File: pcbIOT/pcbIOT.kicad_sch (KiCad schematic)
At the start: 33 parts, among them IC1 NRF52832-QFAA-G-R7, IC2 TPS62842DGRR, J1 Battery power in, J2 Conn_01x08_Socket, J3 Conn_01x03_Pin, J4 Conn_01x06_Socket, J5 Conn_01x06_Socket, X1 32MHz, X2 32.768kHz

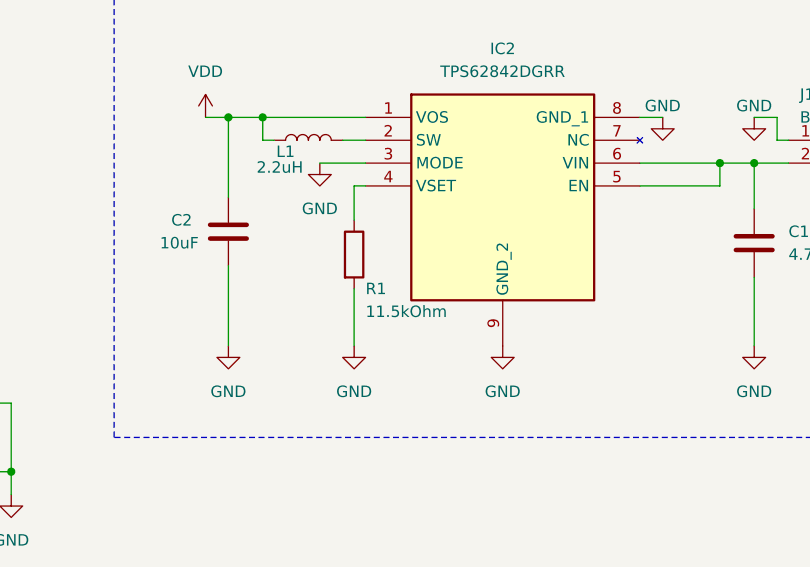
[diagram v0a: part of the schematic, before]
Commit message: pcb bijna af
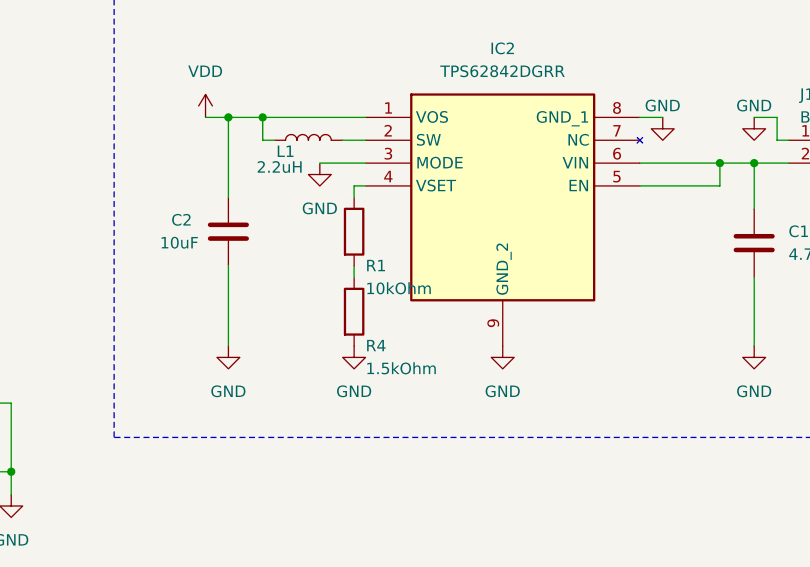
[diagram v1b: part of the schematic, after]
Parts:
- added R4: 1.5kOhm, Resistor_SMD:R_0805_2012Metric_Pad1.20x1.40mm_HandSolder, symbol Device:R
- C1, C10, C11, C12, C13, C14, C15, C2, C3, C4, C5, C6, C7, C8, C9: footprint Capacitor_SMD:C_0603_1608Metric -> Capacitor_SMD:C_0805_2012Metric_Pad1.18x1.45mm_HandSolder
- L4: footprint Inductor_SMD:L_01005_0402Metric_Pad0.57x0.30mm_HandSolder -> Inductor_SMD:L_0805_2012Metric_Pad1.15x1.40mm_HandSolder
- R1: value 11.5kOhm -> 10kOhm; footprint Resistor_SMD:R_0603_1608Metric -> Resistor_SMD:R_0805_2012Metric_Pad1.20x1.40mm_HandSolder
- R2, R3: footprint Resistor_SMD:R_0603_1608Metric -> Resistor_SMD:R_0805_2012Metric_Pad1.20x1.40mm_HandSolder
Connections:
- net GND: now also R4.2; no longer R1.2
- new net: R1.2, R4.1
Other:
- moved on the sheet: R1
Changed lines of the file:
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@@
-    (stroke (width 0) (type default))
-  )
-  (wire (pts (xy 209.55 52.07) (xy 209.55 58.42))
     (stroke (width 0) (type default))
   )
@@
     (stroke (width 0) (type default))
   )
-  (wire (pts (xy 209.55 40.64) (xy 209.55 44.45))
-    (stroke (width 0) (type default))
-  )
   (wire (pts (xy 95.25 58.42) (xy 93.98 58.42))
     (stroke (width 0) (type default))
@@
     (stroke (width 0) (type default))
   )
+  (wire (pts (xy 209.55 49.53) (xy 209.55 50.8))
+    (stroke (width 0) (type default))
+  )
   (wire (pts (xy 212.09 149.86) (xy 214.63 149.86))
     (stroke (width 0) (type default))
@@
   )
   (wire (pts (xy 71.12 93.98) (xy 71.12 83.82))
+    (stroke (width 0) (type default))
+  )
+  (wire (pts (xy 209.55 40.64) (xy 209.55 41.91))
     (stroke (width 0) (type default))
   )
@@
       (effects (font (size 1.27 1.27)) (justify left))
     )
-    (property "Footprint" "Capacitor_SMD:C_0603_1608Metric" (at 74.6252 76.2 0)
+    (property "Footprint" "Capacitor_SMD:C_0805_2012Metric_Pad1.18x1.45mm_HandSolder" (at 74.6252 76.2 0)
       (effects (font (size 1.27 1.27)) hide)
     )
@@
       (effects (font (size 1.27 1.27)) (justify left))
     )
-    (property "Footprint" "Capacitor_SMD:C_0603_1608Metric" (at 158.75 65.7352 0)
+    (property "Footprint" "Capacitor_SMD:C_0805_2012Metric_Pad1.18x1.45mm_HandSolder" (at 158.75 65.7352 0)
       (effects (font (size 1.27 1.27)) hide)
     )
@@
       (effects (font (size 1.27 1.27)) (justify left))
     )
-    (property "Footprint" "Capacitor_SMD:C_0603_1608Metric" (at 40.64 110.1852 0)
+    (property "Footprint" "Capacitor_SMD:C_0805_2012Metric_Pad1.18x1.45mm_HandSolder" (at 40.64 110.1852 0)
       (effects (font (size 1.27 1.27)) hide)
     )
@@
       (effects (font (size 1.27 1.27)) (justify left))
     )
-    (property "Footprint" "Capacitor_SMD:C_0603_1608Metric" (at 158.75 73.3552 0)
+    (property "Footprint" "Capacitor_SMD:C_0805_2012Metric_Pad1.18x1.45mm_HandSolder" (at 158.75 73.3552 0)
       (effects (font (size 1.27 1.27)) hide)
     )
@@
       (effects (font (size 1.27 1.27)) (justify left))
     )
-    (property "Footprint" "Capacitor_SMD:C_0603_1608Metric" (at 40.64 97.4852 0)
+    (property "Footprint" "Capacitor_SMD:C_0805_2012Metric_Pad1.18x1.45mm_HandSolder" (at 40.64 97.4852 0)
       (effects (font (size 1.27 1.27)) hide)
     )
@@
       (effects (font (size 1.27 1.27)) (justify left))
     )
-    (property "Footprint" "Resistor_SMD:R_0603_1608Metric" (at 115.062 48.26 90)
+    (property "Footprint" "Resistor_SMD:R_0805_2012Metric_Pad1.20x1.40mm_HandSolder" (at 115.062 48.26 90)
       (effects (font (size 1.27 1.27)) hide)
     )
@@
       (effects (font (size 1.27 1.27)) (justify left))
     )
-    (property "Footprint" "Capacitor_SMD:C_0603_1608Metric" (at 117.8052 62.23 0)
+    (property "Footprint" "Capacitor_SMD:C_0805_2012Metric_Pad1.18x1.45mm_HandSolder" (at 117.8052 62.23 0)
       (effects (font (size 1.27 1.27)) hide)
     )
@@
       (effects (font (size 1.27 1.27)))
     )
-    (property "Footprint" "Inductor_SMD:L_01005_0402Metric_Pad0.57x0.30mm_HandSolder" (at 149.86 109.22 0)
+    (property "Footprint" "Inductor_SMD:L_0805_2012Metric_Pad1.15x1.40mm_HandSolder" (at 149.86 109.22 0)
       (effects (font (size 1.27 1.27)) hide)
     )
@@
       (effects (font (size 1.27 1.27)) (justify left))
     )
-    (property "Footprint" "Capacitor_SMD:C_0603_1608Metric" (at 69.85 82.8548 0)
+    (property "Footprint" "Capacitor_SMD:C_0805_2012Metric_Pad1.18x1.45mm_HandSolder" (at 69.85 82.8548 0)
       (effects (font (size 1.27 1.27)) hide)
     )
@@
       (effects (font (size 1.27 1.27)) (justify left))
     )
-    (property "Footprint" "Capacitor_SMD:C_0603_1608Metric" (at 107.6452 62.23 0)
+    (property "Footprint" "Capacitor_SMD:C_0805_2012Metric_Pad1.18x1.45mm_HandSolder" (at 107.6452 62.23 0)
       (effects (font (size 1.27 1.27)) hide)
     )
@@
       (effects (font (size 1.27 1.27)) (justify left))
     )
-    (property "Footprint" "Capacitor_SMD:C_0603_1608Metric" (at 196.5452 49.53 0)
+    (property "Footprint" "Capacitor_SMD:C_0805_2012Metric_Pad1.18x1.45mm_HandSolder" (at 196.5452 49.53 0)
       (effects (font (size 1.27 1.27)) hide)
     )
@@
       (effects (font (size 1.27 1.27)) (justify left))
     )
-    (property "Footprint" "Capacitor_SMD:C_0603_1608Metric" (at 127.9652 82.55 0)
+    (property "Footprint" "Capacitor_SMD:C_0805_2012Metric_Pad1.18x1.45mm_HandSolder" (at 127.9652 82.55 0)
       (effects (font (size 1.27 1.27)) hide)
     )
@@
       (effects (font (size 1.27 1.27)) (justify left))
     )
-    (property "Footprint" "Capacitor_SMD:C_0603_1608Metric" (at 254.9652 50.8 0)
+    (property "Footprint" "Capacitor_SMD:C_0805_2012Metric_Pad1.18x1.45mm_HandSolder" (at 254.9652 50.8 0)
       (effects (font (size 1.27 1.27)) hide)
     )
@@
       (effects (font (size 1.27 1.27)) (justify left))
     )
-    (property "Footprint" "Capacitor_SMD:C_0603_1608Metric" (at 75.8952 168.91 0)
+    (property "Footprint" "Capacitor_SMD:C_0805_2012Metric_Pad1.18x1.45mm_HandSolder" (at 75.8952 168.91 0)
       (effects (font (size 1.27 1.27)) hide)
     )
@@
       (effects (font (size 1.27 1.27)) (justify left))
     )
-    (property "Footprint" "Capacitor_SMD:C_0603_1608Metric" (at 140.6652 116.84 0)
+    (property "Footprint" "Capacitor_SMD:C_0805_2012Metric_Pad1.18x1.45mm_HandSolder" (at 140.6652 116.84 0)
       (effects (font (size 1.27 1.27)) hide)
     )
@@
     )
   )
-  (symbol (lib_id "Device:R") (at 209.55 48.26 0) (unit 1)
-    (in_bom yes) (on_board yes) (dnp no)
-    (property "Reference" "R1" (at 210.82 52.07 0)
-      (effects (font (size 1.27 1.27)) (justify left))
-    )
-    (property "Value" "11.5kOhm" (at 210.82 54.61 0)
-      (effects (font (size 1.27 1.27)) (justify left))
-    )
-    (property "Footprint" "Resistor_SMD:R_0603_1608Metric" (at 207.772 48.26 90)
-      (effects (font (size 1.27 1.27)) hide)
-    )
-    (property "Datasheet" "~" (at 209.55 48.26 0)
+  (symbol (lib_id "Device:R") (at 209.55 45.72 0) (unit 1)
+    (in_bom yes) (on_board yes) (dnp no)
+    (property "Reference" "R1" (at 210.82 49.53 0)
+      (effects (font (size 1.27 1.27)) (justify left))
+    )
+    (property "Value" "10kOhm" (at 210.82 52.07 0)
+      (effects (font (size 1.27 1.27)) (justify left))
+    )
+    (property "Footprint" "Resistor_SMD:R_0805_2012Metric_Pad1.20x1.40mm_HandSolder" (at 207.772 45.72 90)
+      (effects (font (size 1.27 1.27)) hide)
+    )
+    (property "Datasheet" "~" (at 209.55 45.72 0)
       (effects (font (size 1.27 1.27)) hide)
     )
@@
       (effects (font (size 1.27 1.27)) (justify left))
     )
-    (property "Footprint" "Capacitor_SMD:C_0603_1608Metric" (at 94.9452 58.42 0)
+    (property "Footprint" "Capacitor_SMD:C_0805_2012Metric_Pad1.18x1.45mm_HandSolder" (at 94.9452 58.42 0)
       (effects (font (size 1.27 1.27)) hide)
     )
@@
     )
   )
+  (symbol (lib_id "Device:R") (at 209.55 54.61 0) (unit 1)
+    (in_bom yes) (on_board yes) (dnp no)
+    (property "Reference" "R4" (at 210.82 58.42 0)
+      (effects (font (size 1.27 1.27)) (justify left))
+    )
+    (property "Value" "1.5kOhm" (at 210.82 60.96 0)
+      (effects (font (size 1.27 1.27)) (justify left))
+    )
+    (property "Footprint" "Resistor_SMD:R_0805_2012Metric_Pad1.20x1.40mm_HandSolder" (at 207.772 54.61 90)
+      (effects (font (size 1.27 1.27)) hide)
+    )
+    (property "Datasheet" "~" (at 209.55 54.61 0)
+      (effects (font (size 1.27 1.27)) hide)
+    )
+    (pin "1")
+    (pin "2")
+    (instances
+      (project "pcbIOT"
+        (path "/79d26ad8-5789-46cf-878f-e49e2e4d86d0"
+          (reference "R4") (unit 1)
+        )
+      )
+    )
+  )
   (symbol (lib_id "power:GND") (at 34.29 113.03 0) (unit 1)
     (in_bom yes) (on_board yes) (dnp no) (fields_autoplaced)
@@
       (effects (font (size 1.27 1.27)) (justify left))
     )
-    (property "Footprint" "Capacitor_SMD:C_0603_1608Metric" (at 154.94 94.9452 0)
+    (property "Footprint" "Capacitor_SMD:C_0805_2012Metric_Pad1.18x1.45mm_HandSolder" (at 154.94 94.9452 0)
       (effects (font (size 1.27 1.27)) hide)
     )
@@
       (effects (font (size 1.27 1.27)) (justify left))
     )
-    (property "Footprint" "Resistor_SMD:R_0603_1608Metric" (at 104.902 48.26 90)
-      (effects (font (size 1.27 1.27)) hide)
-    )
+    (property "Footprint" "Resistor_SMD:R_0805_2012Metric_Pad1.20x1.40mm_HandSolder" (at 104.902 48.26 90)
+      (effects (font (size 1.27 1.27)) hide)
+    )

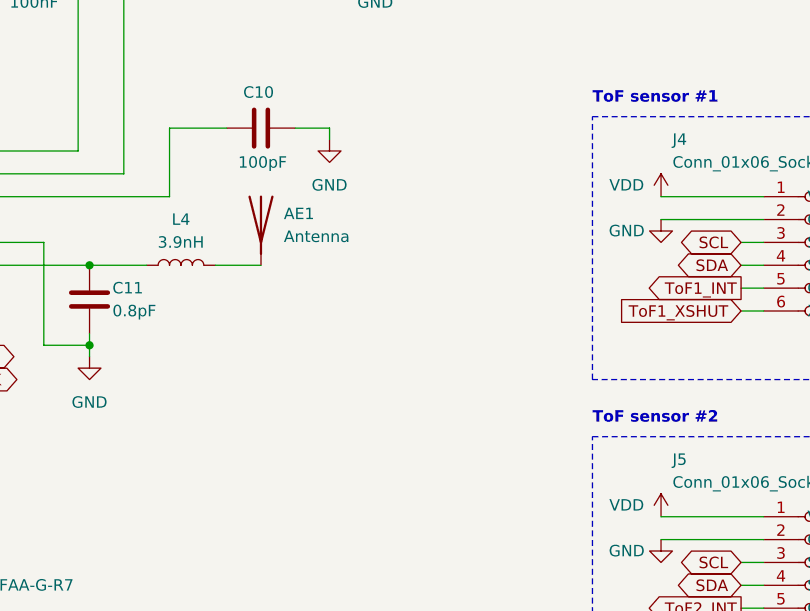
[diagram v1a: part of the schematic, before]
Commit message: Schema update
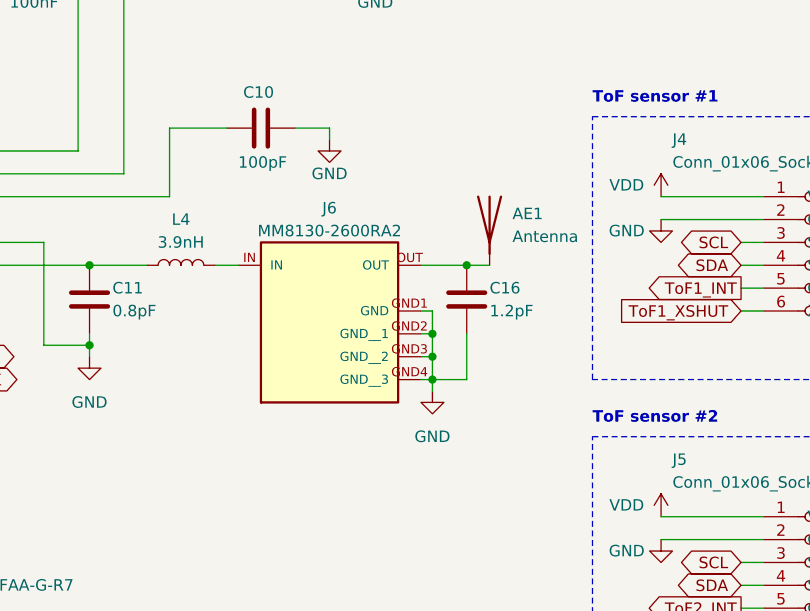
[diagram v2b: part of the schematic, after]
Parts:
- added C16: 1.2pF, Capacitor_SMD:C_0805_2012Metric_Pad1.18x1.45mm_HandSolder, symbol Device:C
- added J6: MM8130-2600RA2, footprints:MURATA_MM8130-2600RA2, symbol MM8130-2600RA2:MM8130-2600RA2
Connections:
- net GND: now also C16.2, J6.GND1 (GND), J6.GND2 (GND__1), J6.GND3 (GND__2), J6.GND4 (GND__3)
- net at L4.2: now also J6.IN; no longer AE1.1 (A)
- new net: AE1.1 (A), C16.1, J6.OUT
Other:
- moved on the sheet: AE1
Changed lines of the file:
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@@
   (junction (at 250.19 38.1) (diameter 0) (color 0 0 0 0)
   )
+  (junction (at 177.8 119.38) (diameter 0) (color 0 0 0 0)
+  )
   (junction (at 171.45 72.39) (diameter 0) (color 0 0 0 0)
   )
@@
   (junction (at 34.29 109.22) (diameter 0) (color 0 0 0 0)
   )
+  (junction (at 177.8 121.92) (diameter 0) (color 0 0 0 0)
+  )
   (junction (at 139.7 109.22) (diameter 0) (color 0 0 0 0)
   )
@@
   (junction (at 52.07 109.22) (diameter 0) (color 0 0 0 0)
   )
+  (junction (at 181.61 109.22) (diameter 0) (color 0 0 0 0)
+  )
   (junction (at 195.58 33.02) (diameter 0) (color 0 0 0 0)
   )
@@
   )
   (junction (at 93.98 49.53) (diameter 0) (color 0 0 0 0)
+  )
+  (junction (at 177.8 116.84) (diameter 0) (color 0 0 0 0)
   )
   (junction (at 139.7 118.11) (diameter 0) (color 0 0 0 0)
@@
     (stroke (width 0) (type default))
   )
+  (wire (pts (xy 177.8 116.84) (xy 177.8 119.38))
+    (stroke (width 0) (type default))
+  )
   (wire (pts (xy 40.64 96.52) (xy 34.29 96.52))
     (stroke (width 0) (type default))
@@
     (stroke (width 0) (type default))
   )
+  (wire (pts (xy 181.61 109.22) (xy 184.15 109.22))
+    (stroke (width 0) (type default))
+  )
   (wire (pts (xy 264.16 143.51) (xy 265.43 143.51))
     (stroke (width 0) (type default))
@@
     (stroke (width 0) (type default))
   )
+  (wire (pts (xy 153.67 109.22) (xy 156.21 109.22))
+    (stroke (width 0) (type default))
+  )
   (wire (pts (xy 92.71 71.12) (xy 92.71 58.42))
     (stroke (width 0) (type default))
@@
     (stroke (width 0) (type default))
   )
+  (wire (pts (xy 176.53 121.92) (xy 177.8 121.92))
+    (stroke (width 0) (type default))
+  )
   (wire (pts (xy 116.84 52.07) (xy 116.84 53.34))
     (stroke (width 0) (type default))
@@
     (stroke (width 0) (type default))
   )
+  (wire (pts (xy 177.8 121.92) (xy 177.8 123.19))
+    (stroke (width 0) (type default))
+  )
   (wire (pts (xy 110.49 160.02) (xy 110.49 162.56))
     (stroke (width 0) (type default))
@@
     (stroke (width 0) (type default))
   )
+  (wire (pts (xy 181.61 121.92) (xy 177.8 121.92))
+    (stroke (width 0) (type default))
+  )
+  (wire (pts (xy 181.61 116.84) (xy 181.61 121.92))
+    (stroke (width 0) (type default))
+  )
+  (wire (pts (xy 176.53 119.38) (xy 177.8 119.38))
+    (stroke (width 0) (type default))
+  )
   (wire (pts (xy 95.25 58.42) (xy 93.98 58.42))
     (stroke (width 0) (type default))
@@
     (stroke (width 0) (type default))
   )
+  (wire (pts (xy 177.8 119.38) (xy 177.8 121.92))
+    (stroke (width 0) (type default))
+  )
   (wire (pts (xy 110.49 48.26) (xy 110.49 53.34))
     (stroke (width 0) (type default))
@@
     (stroke (width 0) (type default))
   )
+  (wire (pts (xy 176.53 114.3) (xy 177.8 114.3))
+    (stroke (width 0) (type default))
+  )
   (wire (pts (xy 106.68 43.18) (xy 106.68 44.45))
     (stroke (width 0) (type default))
@@
     (stroke (width 0) (type default))
   )
+  (wire (pts (xy 176.53 116.84) (xy 177.8 116.84))
+    (stroke (width 0) (type default))
+  )
   (wire (pts (xy 267.97 107.95) (xy 270.51 107.95))
     (stroke (width 0) (type default))
@@
     (stroke (width 0) (type default))
   )
+  (wire (pts (xy 177.8 114.3) (xy 177.8 116.84))
+    (stroke (width 0) (type default))
+  )
   (wire (pts (xy 240.03 138.43) (xy 241.3 138.43))
     (stroke (width 0) (type default))
@@
     (stroke (width 0) (type default))
   )
-  (wire (pts (xy 153.67 109.22) (xy 158.75 109.22))
+  (wire (pts (xy 176.53 109.22) (xy 181.61 109.22))
     (stroke (width 0) (type default))
   )
@@
         (path "/79d26ad8-5789-46cf-878f-e49e2e4d86d0"
           (reference "#PWR011") (unit 1)
+        )
+      )
+    )
+  )
+  (symbol (lib_id "MM8130-2600RA2:MM8130-2600RA2") (at 166.37 111.76 0) (unit 1)
+    (in_bom yes) (on_board yes) (dnp no)
+    (property "Reference" "J6" (at 166.37 102.87 0)
+      (effects (font (size 1.27 1.27)))
+    )
+    (property "Value" "MM8130-2600RA2" (at 166.37 105.41 0)
+      (effects (font (size 1.27 1.27)))
+    )
+    (property "Footprint" "footprints:MURATA_MM8130-2600RA2" (at 166.37 111.76 0)
+      (effects (font (size 1.27 1.27)) (justify bottom) hide)
+    )
+    (property "Datasheet" "" (at 166.37 111.76 0)
+      (effects (font (size 1.27 1.27)) hide)
+    )
+    (property "MANUFACTURER" "MURATA" (at 166.37 111.76 0)
+      (effects (font (size 1.27 1.27)) (justify bottom) hide)
+    )
+    (pin "GND1")
+    (pin "GND2")
+    (pin "GND3")
+    (pin "GND4")
+    (pin "IN")
+    (pin "OUT")
+    (instances
+      (project "pcbIOT"
+        (path "/79d26ad8-5789-46cf-878f-e49e2e4d86d0"
+          (reference "J6") (unit 1)
         )
       )
@@
   )
   (symbol (lib_id "power:GND") (at 166.37 95.25 0) (unit 1)
-    (in_bom yes) (on_board yes) (dnp no) (fields_autoplaced)
+    (in_bom yes) (on_board yes) (dnp no)
     (property "Reference" "#PWR025" (at 166.37 101.6 0)
       (effects (font (size 1.27 1.27)) hide)
     )
-    (property "Value" "GND" (at 166.37 100.33 0)
+    (property "Value" "GND" (at 166.37 99.06 0)
       (effects (font (size 1.27 1.27)))
     )
@@
     )
   )
+  (symbol (lib_id "power:GND") (at 177.8 123.19 0) (unit 1)
+    (in_bom yes) (on_board yes) (dnp no) (fields_autoplaced)
+    (property "Reference" "#PWR038" (at 177.8 129.54 0)
+      (effects (font (size 1.27 1.27)) hide)
+    )
+    (property "Value" "GND" (at 177.8 128.27 0)
+      (effects (font (size 1.27 1.27)))
+    )
+    (property "Footprint" "" (at 177.8 123.19 0)
+      (effects (font (size 1.27 1.27)) hide)
+    )
+    (property "Datasheet" "" (at 177.8 123.19 0)
+      (effects (font (size 1.27 1.27)) hide)
+    )
+    (pin "1")
+    (instances
+      (project "pcbIOT"
+        (path "/79d26ad8-5789-46cf-878f-e49e2e4d86d0"
+          (reference "#PWR038") (unit 1)
+        )
+      )
+    )
+  )
   (symbol (lib_id "power:VDD") (at 203.2 101.6 0) (unit 1)
     (in_bom yes) (on_board yes) (dnp no)
@@
     )
   )
-  (symbol (lib_id "Device:Antenna") (at 158.75 104.14 0) (unit 1)
+  (symbol (lib_id "Device:Antenna") (at 184.15 104.14 0) (unit 1)
     (in_bom yes) (on_board yes) (dnp no) (fields_autoplaced)
-    (property "Reference" "AE1" (at 161.29 103.505 0)
-      (effects (font (size 1.27 1.27)) (justify left))
-    )
-    (property "Value" "Antenna" (at 161.29 106.045 0)
-      (effects (font (size 1.27 1.27)) (justify left))
-    )
-    (property "Footprint" "RF_Antenna:Texas_SWRA117D_2.4GHz_Right" (at 158.75 104.14 0)
-      (effects (font (size 1.27 1.27)) hide)
-    )
-    (property "Datasheet" "~" (at 158.75 104.14 0)
+    (property "Reference" "AE1" (at 186.69 103.505 0)
+      (effects (font (size 1.27 1.27)) (justify left))
+    )
+    (property "Value" "Antenna" (at 186.69 106.045 0)
+      (effects (font (size 1.27 1.27)) (justify left))
+    )
+    (property "Footprint" "RF_Antenna:Texas_SWRA117D_2.4GHz_Right" (at 184.15 104.14 0)
+      (effects (font (size 1.27 1.27)) hide)
+    )
+    (property "Datasheet" "~" (at 184.15 104.14 0)
       (effects (font (size 1.27 1.27)) hide)
     )
@@
         )
       )
+    )
+  )
+  (symbol (lib_id "Device:C") (at 181.61 113.03 0) (unit 1)
+    (in_bom yes) (on_board yes) (dnp no)
+    (property "Reference" "C16" (at 184.15 111.76 0)
+      (effects (font (size 1.27 1.27)) (justify left))
+    )
+    (property "Value" "1.2pF" (at 184.15 114.3 0)
+      (effects (font (size 1.27 1.27)) (justify left))
+    )
+    (property "Footprint" "Capacitor_SMD:C_0805_2012Metric_Pad1.18x1.45mm_HandSolder" (at 182.5752 116.84 0)
+      (effects (font (size 1.27 1.27)) hide)
+    )
+    (property "Datasheet" "~" (at 181.61 113.03 0)
+      (effects (font (size 1.27 1.27)) hide)
+    )
+    (pin "1")
+    (pin "2")
+    (instances
+      (project "pcbIOT"
+        (path "/79d26ad8-5789-46cf-878f-e49e2e4d86d0"
+          (reference "C16") (unit 1)
+        )
+      )
